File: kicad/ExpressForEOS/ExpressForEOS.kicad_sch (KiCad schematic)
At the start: 10 parts, among them J1 Conn_02x17_Counter_Clockwise, U11 74LS156, U12 74LS156, U13 74LS373, U14 ICM7218BIPI, U15 MAX150BCPP, U6 74LS138, U7 74LS374, U8 74LS374, U9 74LS245

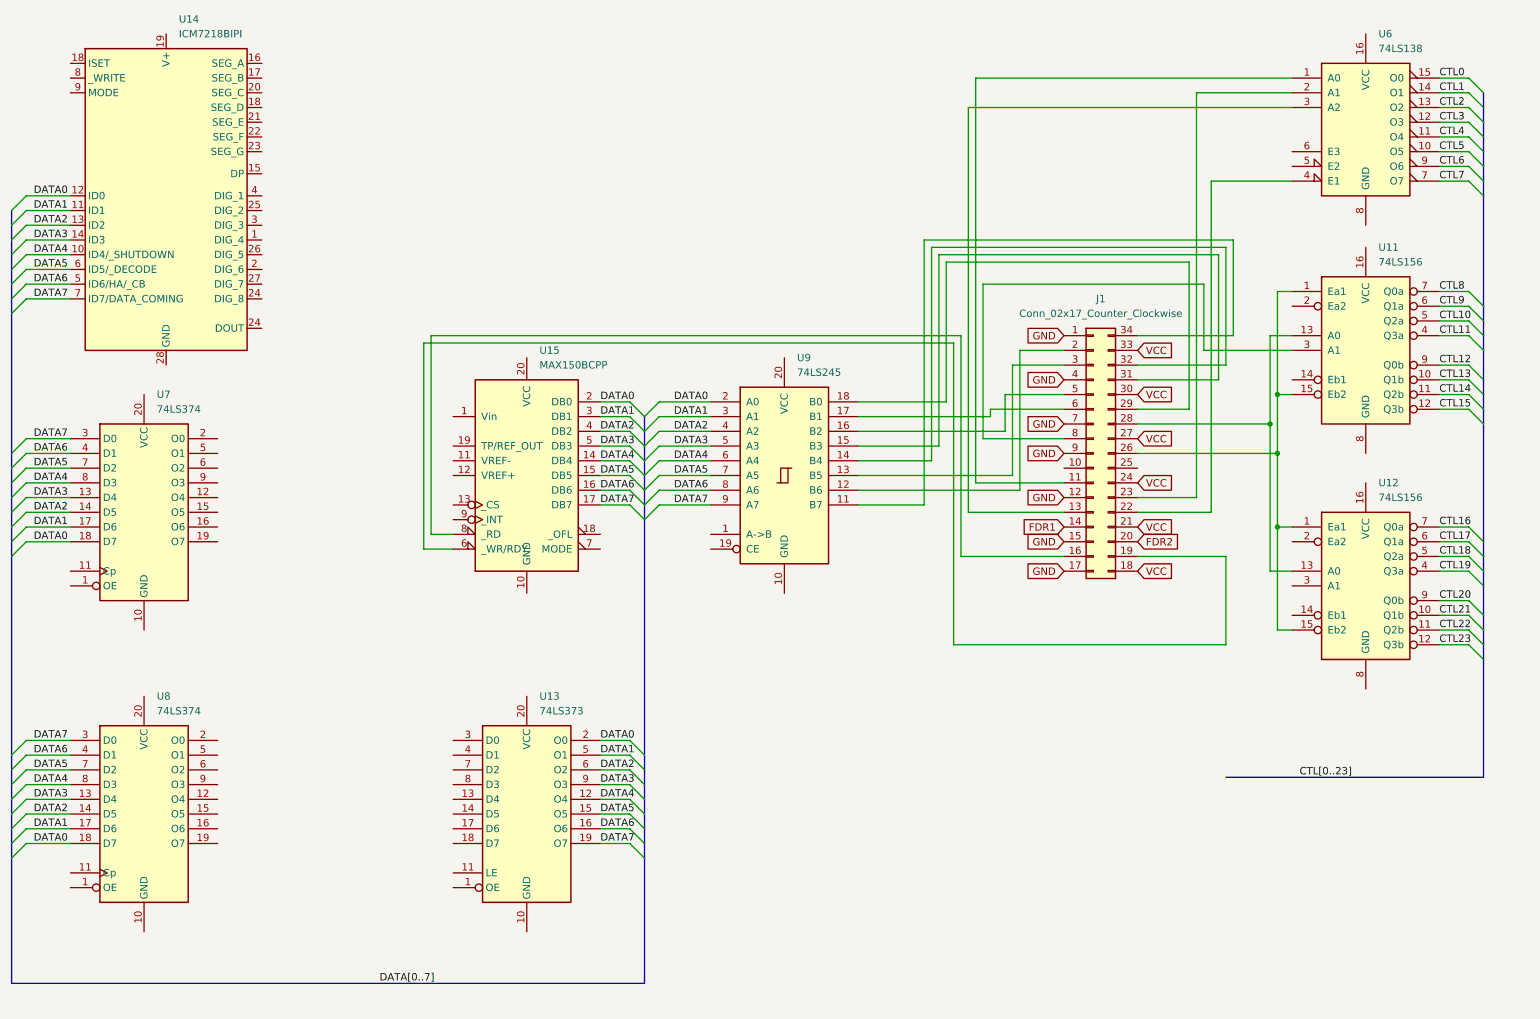
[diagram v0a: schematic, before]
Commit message: more schematic updates, another datasheet
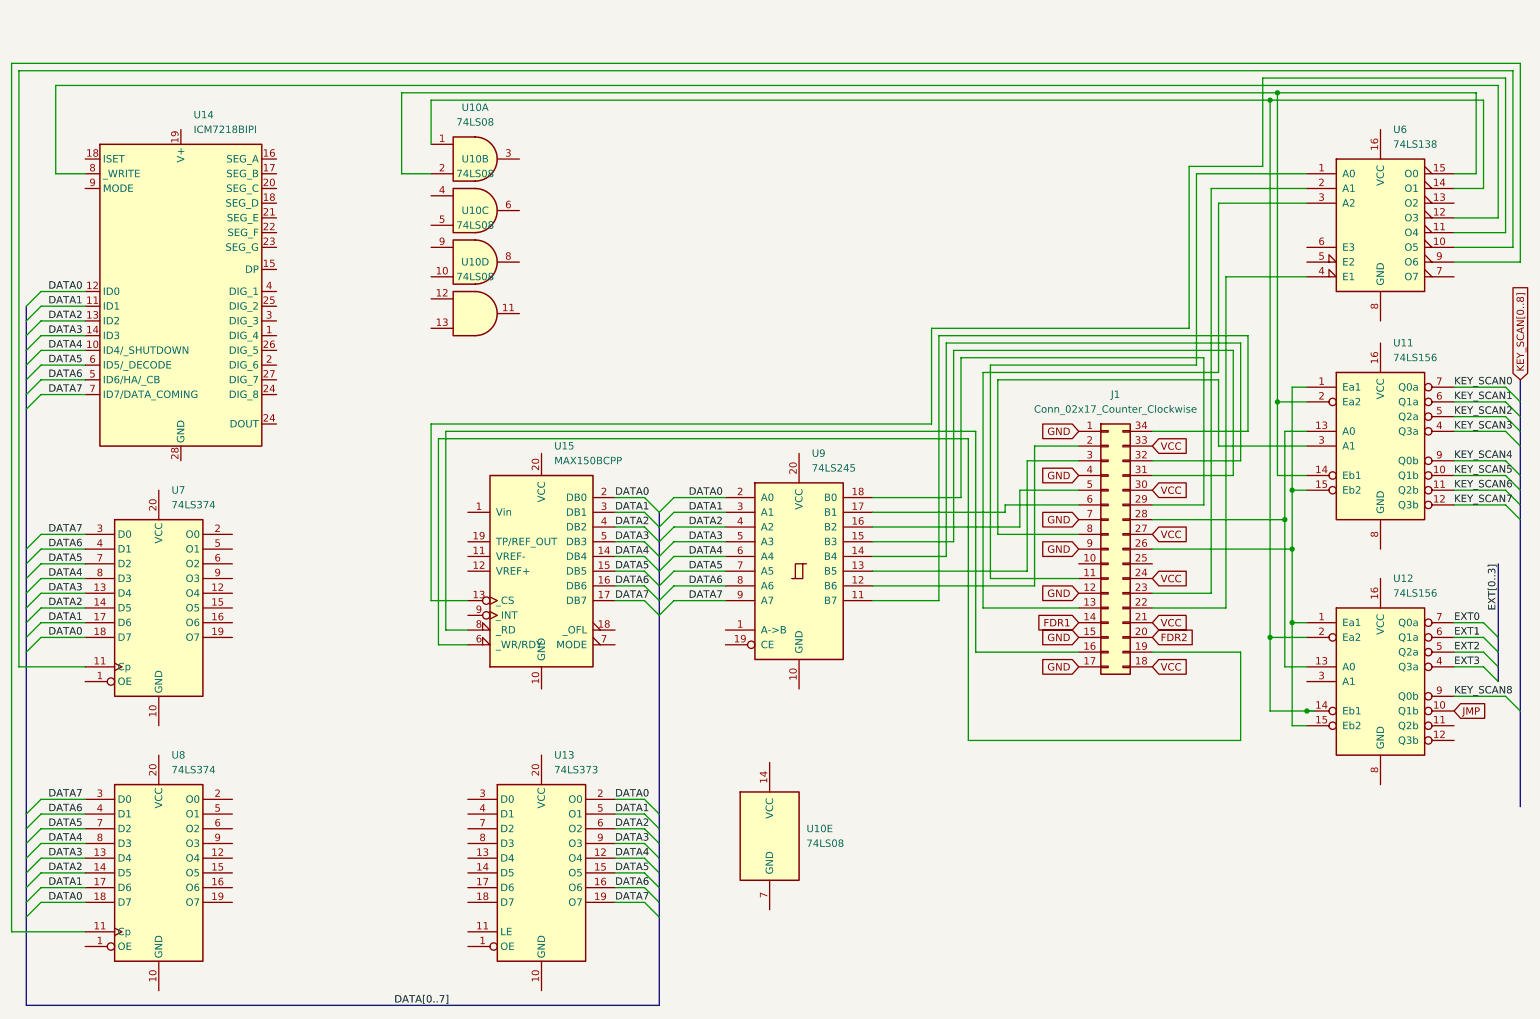
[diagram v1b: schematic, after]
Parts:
- added U10: 74LS08, symbol 74xx:74LS08
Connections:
- net CTL0 is gone; now on an unnamed net: U6.15 (O0)
- net CTL1 is gone; now on an unnamed net: U6.14 (O1)
- net CTL3 is gone; now on an unnamed net: U6.12 (O3)
- net CTL4 is gone; now on an unnamed net: U6.11 (O4)
- net CTL5 is gone; now on an unnamed net: U6.10 (O5)
- net CTL6 is gone; now on an unnamed net: U6.9 (O6)
- net at U11.14 (Eb1): now also U11.2 (Ea2), U10.2
- net at U12.14 (Eb1): now also U12.2 (Ea2), U10.1
- net CTL10 renamed KEY_SCAN2
- net CTL11 renamed KEY_SCAN3
- net CTL12 renamed KEY_SCAN4
- net CTL13 renamed KEY_SCAN5
- net CTL14 renamed KEY_SCAN6
- net CTL15 renamed KEY_SCAN7
- net CTL16 renamed EXT0
- net CTL17 renamed EXT1
- net CTL18 renamed EXT2
- net CTL19 renamed EXT3
- net CTL2: no longer names the net of U6.13 (O2)
- net CTL20 renamed KEY_SCAN8
- net CTL21 renamed JMP
- net CTL22: no longer names the net of U12.11 (Q2b)
- net CTL23: no longer names the net of U12.12 (Q3b)
- net CTL7: no longer names the net of U6.7 (O7)
- net CTL8 renamed KEY_SCAN0
- net CTL9 renamed KEY_SCAN1
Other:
- moved on the sheet: J1, U11, U12, U13, U14, U15, U6, U7, U8, U9
